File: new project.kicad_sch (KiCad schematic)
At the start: 12 parts, among them J1 LED 0.170amps, J2 Tractive Battery

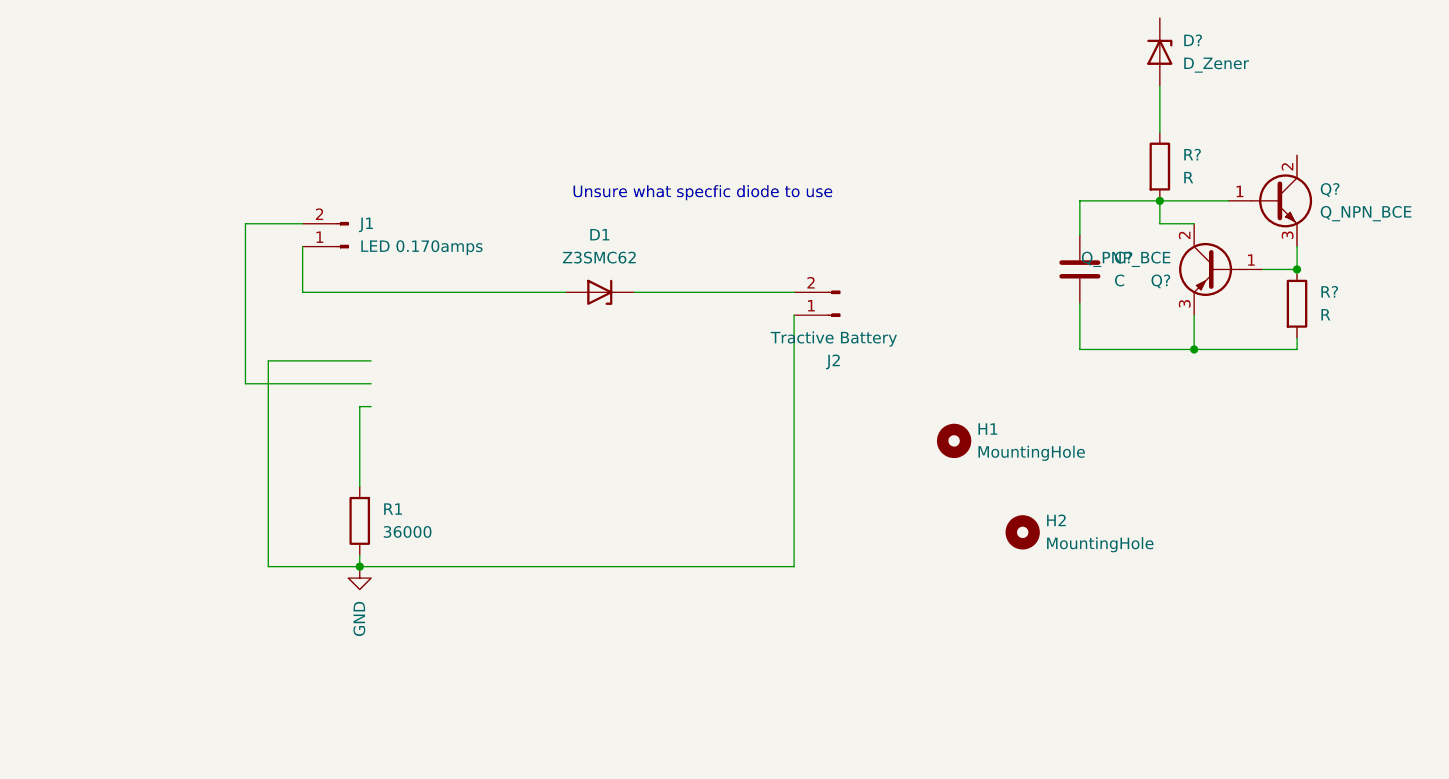
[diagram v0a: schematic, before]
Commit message: w
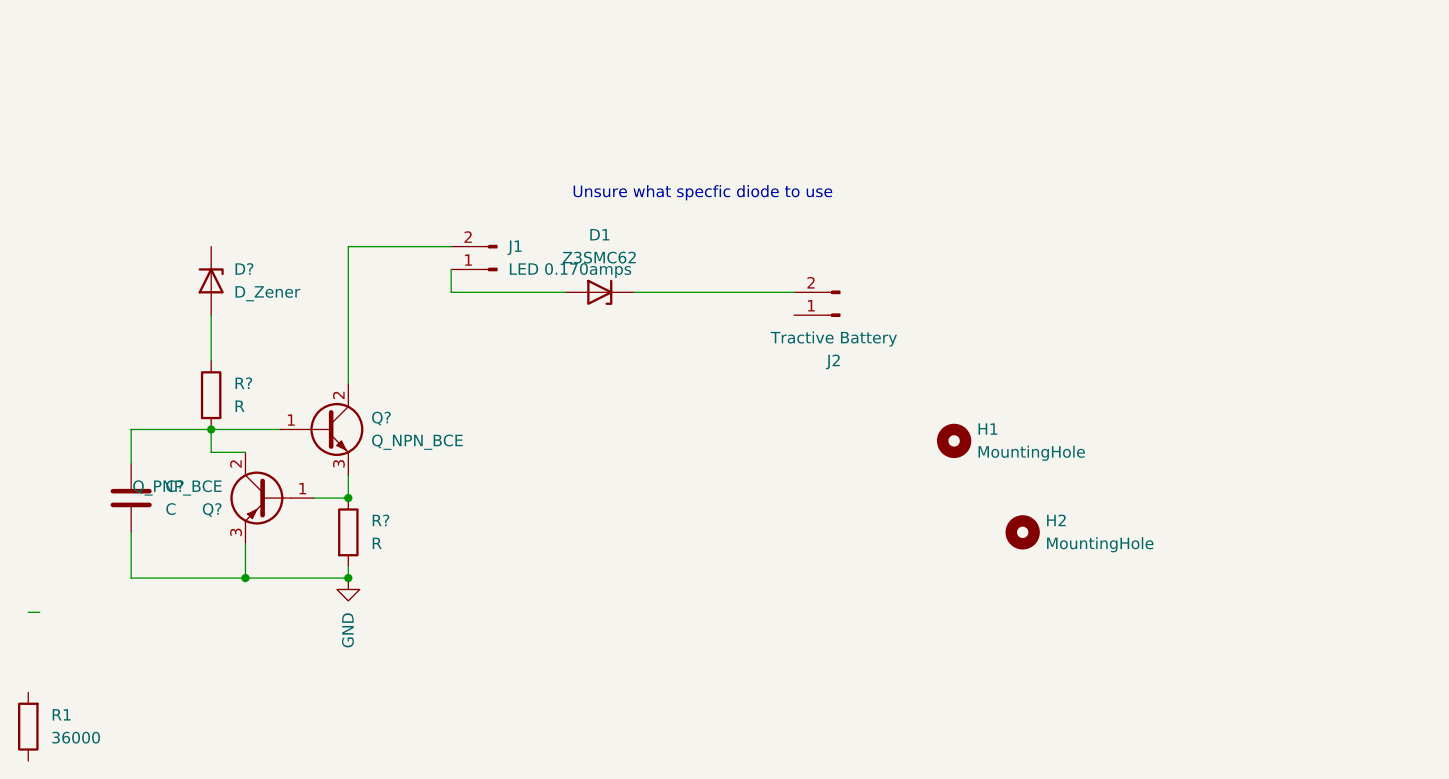
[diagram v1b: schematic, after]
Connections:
- net GND: now also C?.2, Q?.3 (E), R?.2; no longer J2.1 (Pin_1), R1.1
- net at Q?.2 (C): now also J1.2 (Pin_2)
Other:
- moved on the sheet: C?, D?, J1, Q?, R1, R?
